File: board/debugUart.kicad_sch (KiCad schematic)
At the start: 17 parts, among them J2 629105150521, U7 CP2102N-Axx-xQFN20

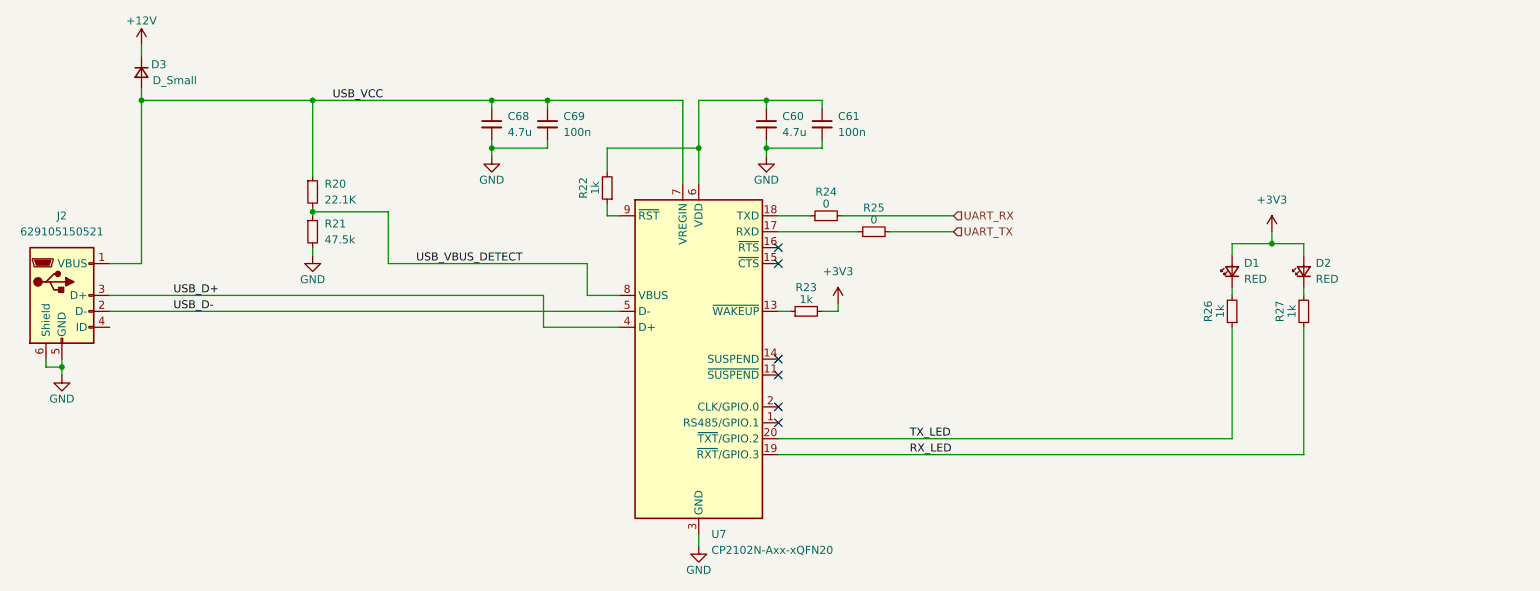
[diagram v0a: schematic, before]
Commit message: update layout
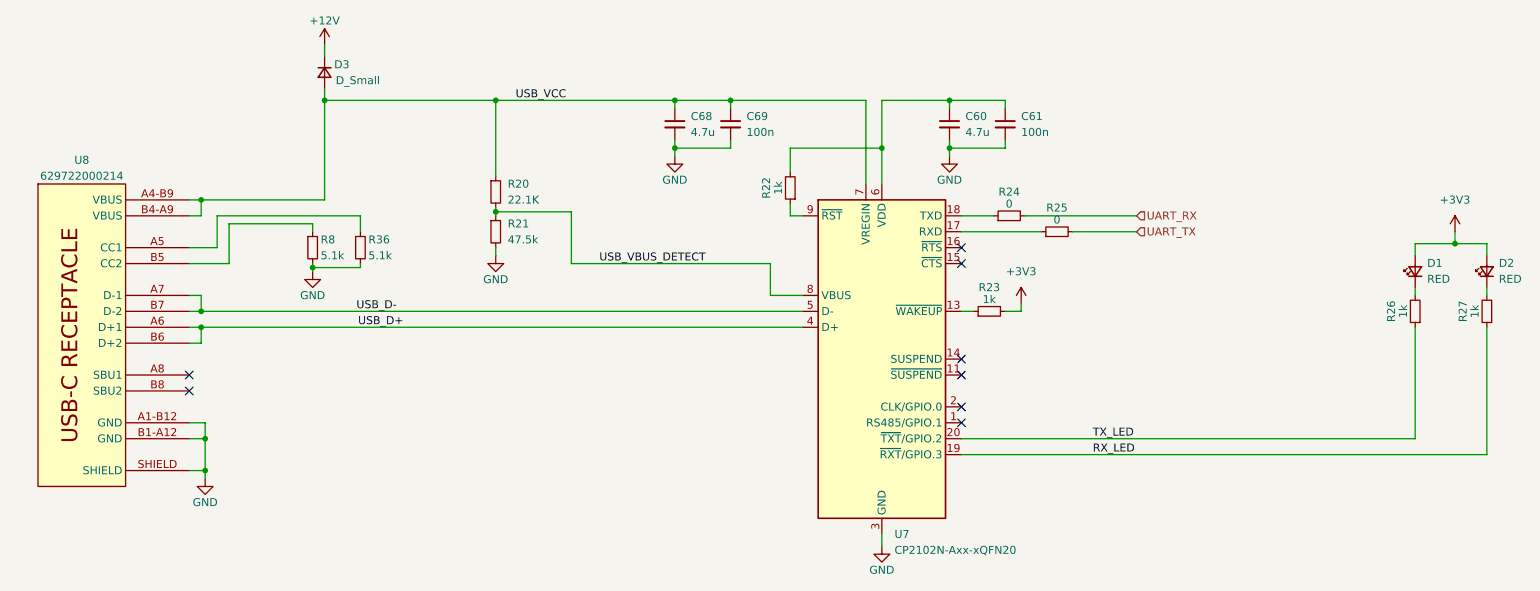
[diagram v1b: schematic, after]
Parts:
- removed J2: 629105150521, v3s:629105150521, symbol Connector:USB_B_Micro
- added R36, R8: 5.1k, Resistor_SMD:R_0603_1608Metric, symbol Device:R_Small
- added U8: 629722000214, v3s:629722000214, symbol v3s:629722000214
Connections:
- net GND: now also R36.2, R8.2, U8.A1-B12 (GND), U8.B1-A12 (GND), U8.SHIELD
- net USB_D+: now also U8.A6 (D+1), U8.B6 (D+2)
- net USB_D-: now also U8.A7 (D-1), U8.B7 (D-2)
- net USB_VCC: now also U8.A4-B9 (VBUS), U8.B4-A9 (VBUS)
- new net: R36.1, U8.A5 (CC1)
- new net: R8.1, U8.B5 (CC2)
- no-connect marks 6 -> 8
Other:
- moved on the sheet: C60, C61, C68, C69, D1, D2, D3, R20, R21, R22, R23, R24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

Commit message: updates, finish layout, remove usb-uart
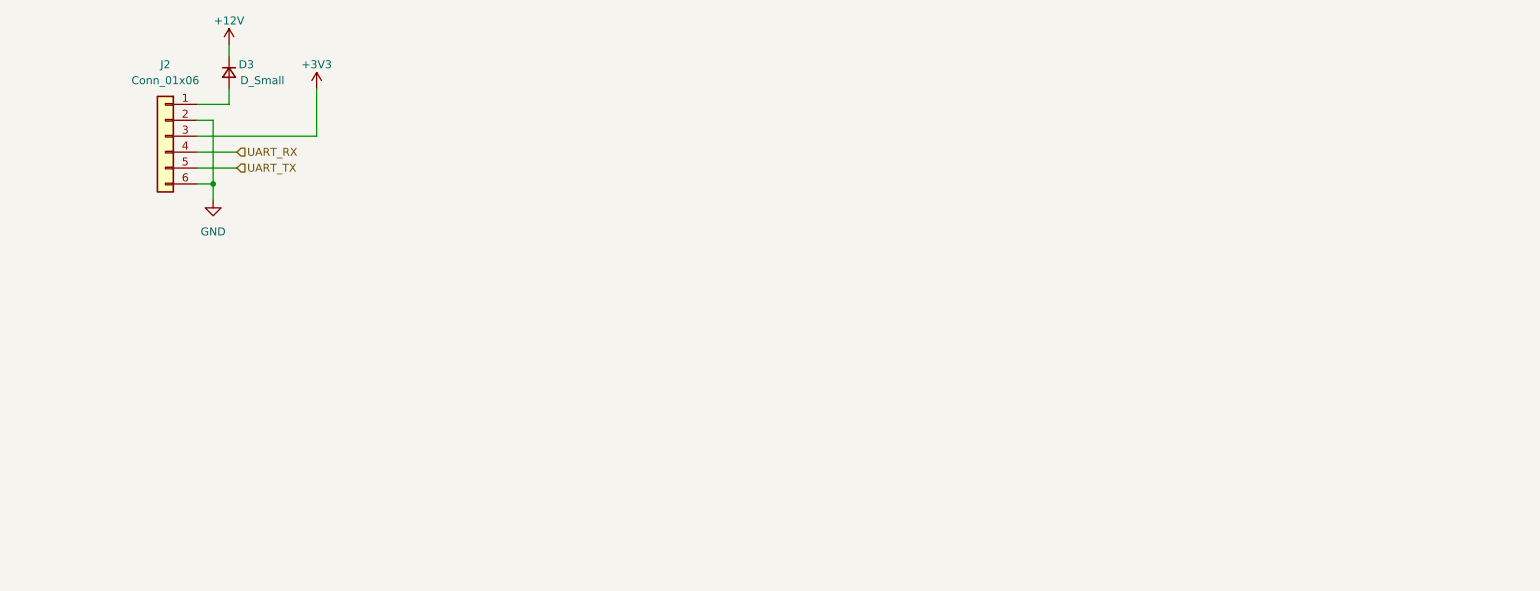
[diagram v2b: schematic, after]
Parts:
- removed C60, C68: 4.7u, Capacitor_SMD:C_0603_1608Metric, symbol Device:C_Small
- removed C61, C69: 100n, Capacitor_SMD:C_0603_1608Metric, symbol Device:C_Small
- removed D1, D2: RED, LED_SMD:LED_0805_2012Metric, symbol Device:LED_Small
- removed R20: 22.1K, Resistor_SMD:R_0603_1608Metric, symbol Device:R_Small
- removed R21: 47.5k, Resistor_SMD:R_0603_1608Metric, symbol Device:R_Small
- removed R22, R23, R26, R27: 1k, Resistor_SMD:R_0603_1608Metric, symbol Device:R_Small
- removed R24, R25: 0, Resistor_SMD:R_0603_1608Metric, symbol Device:R_Small
- removed R36, R8: 5.1k, Resistor_SMD:R_0603_1608Metric, symbol Device:R_Small
- removed U7: CP2102N-Axx-xQFN20, Package_DFN_QFN:SiliconLabs_QFN-20-1EP_3x3mm_P0.5mm_EP1.8x1.8mm, symbol Interface_USB:CP2102N-Axx-xQFN20
- removed U8: 629722000214, v3s:629722000214, symbol v3s:629722000214
- added J2: Conn_01x06, Connector_JST:JST_PH_B6B-PH-K_1x06_P2.00mm_Vertical, symbol Connector_Generic:Conn_01x06
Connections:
- net +3V3: now also J2.3 (Pin_3)
- net GND: now also J2.2 (Pin_2), J2.6 (Pin_6)
- net UART_RX: now also J2.4 (Pin_4)
- net UART_TX: now also J2.5 (Pin_5)
- net USB_VCC: no longer names the net of D3.2 (A)
- net USB_VCC: now also J2.1 (Pin_1)
- no-connect marks 8 -> 0
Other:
- moved on the sheet: D3
